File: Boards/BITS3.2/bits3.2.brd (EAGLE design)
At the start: 45 x 49.7 mm, 33 parts, among them U1 LMR16020, X1 53261-04, X2 53398-10

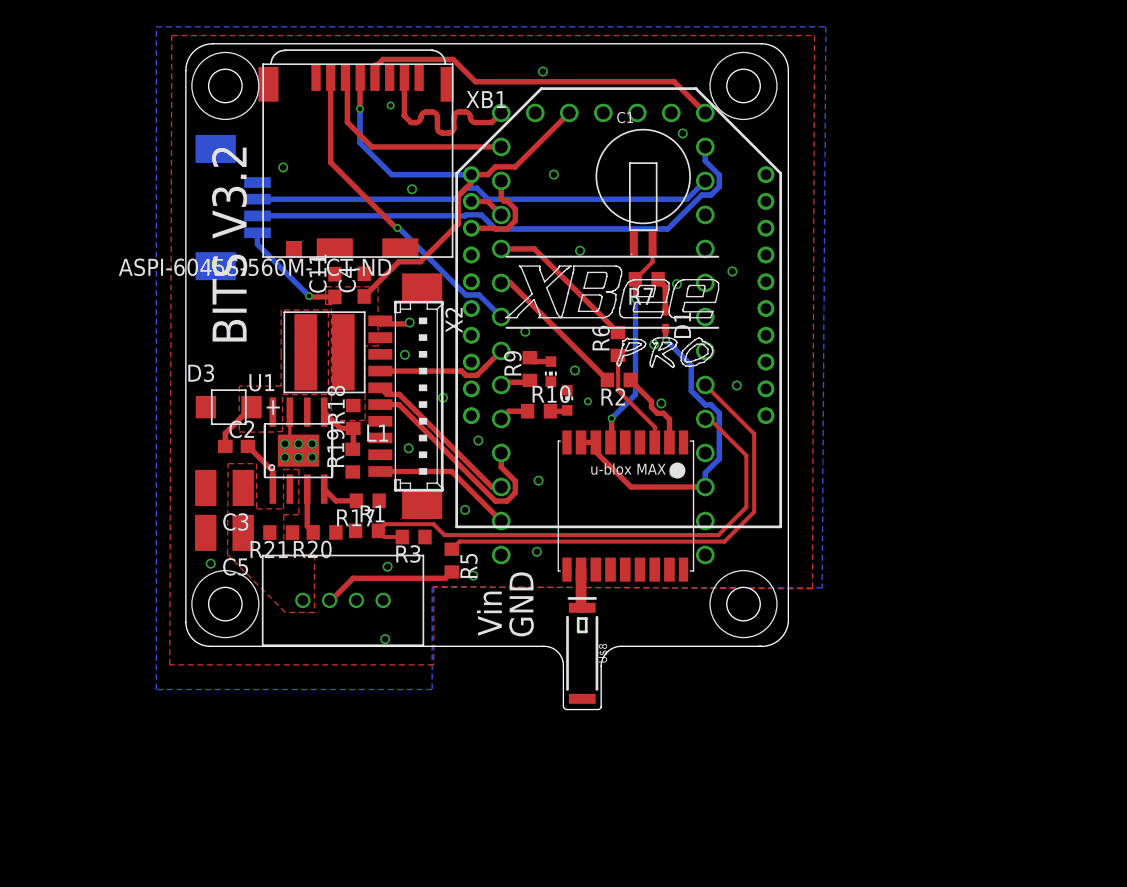
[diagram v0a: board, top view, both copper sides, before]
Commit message: Finalizing BITS v3.2
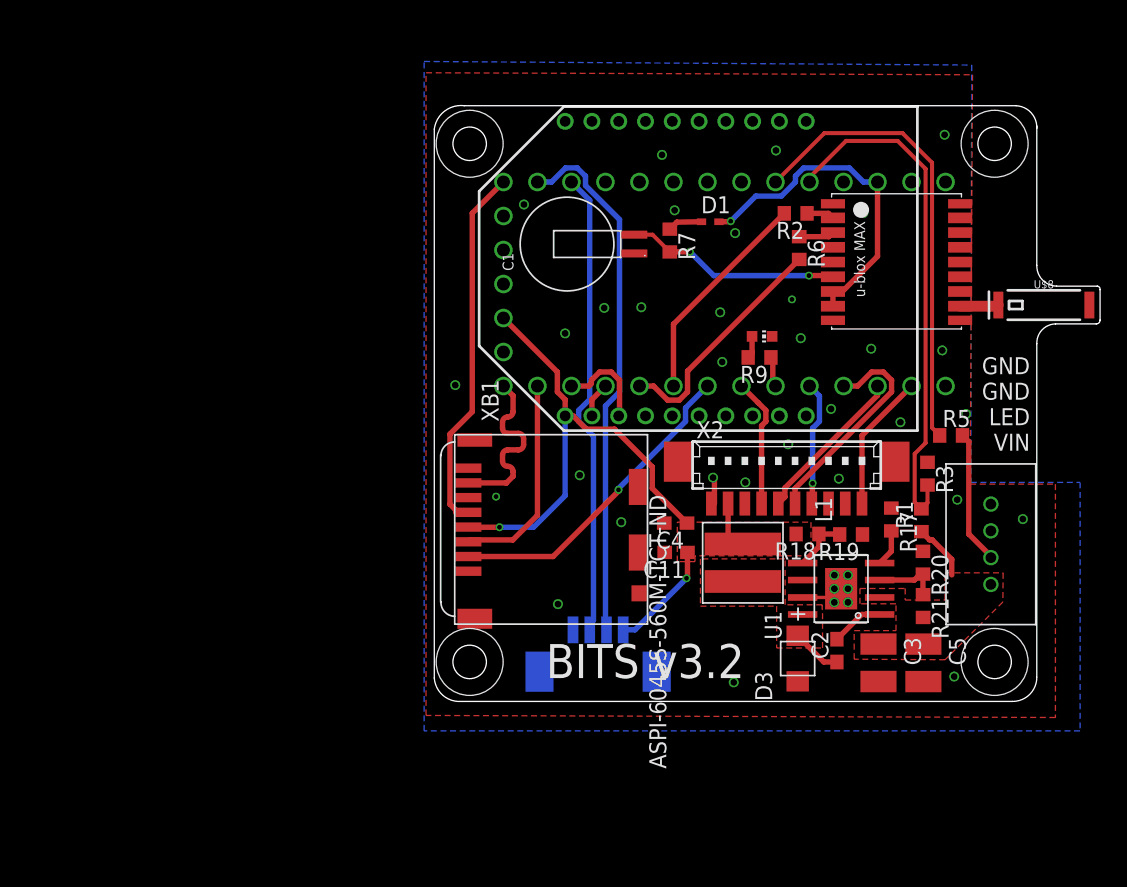
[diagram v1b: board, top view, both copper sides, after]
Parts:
- removed LED2: Green, led:CHIP-LED0603
- removed R10: 470, resistor:R0603
- moved C5 53.1 mm to (55.3, -1.24), turned to 270 degrees
- moved C3 50.6 mm to (51.9, -1.23), turned to 270 degrees
- moved U$1 48.6 mm to (60.3, 7.62), turned to 90 degrees
- moved R21 48.3 mm to (55.3, 3.01), turned to 270 degrees
- moved C2 47.4 mm to (48.8, -0.32), turned to 90 degrees
- moved D3 46.5 mm to (45.9, -0.92), turned to 90 degrees
- moved R20 44.7 mm to (55.3, 6.24), turned to 270 degrees
- moved X1 44.0 mm to (31.0, -1.27), turned to 180 degrees
- moved U$8 43.2 mm to (64.3, 25.5), turned to 0 degrees
- moved U1 41.8 mm to (49.1, 4.30), turned to 90 degrees
- moved R1 41.4 mm to (55.1, 9.41), turned to 90 degrees
- moved R17 39.1 mm to (52.9, 9.47), turned to 270 degrees
- moved R3 38.7 mm to (55.6, 12.9), turned to 270 degrees
- moved R5 38.4 mm to (57.4, 15.7), turned to 0 degrees
- moved R19 37.6 mm to (49.9, 8.35), turned to 180 degrees
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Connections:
- removed net LED2: R10.1, U$2.3
- removed net N$5: LED2.A, R10.2
- net GND: no longer LED2.C
- net NETAV: now also U$2.3
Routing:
- net NETAV: track 0.00 -> 9.32 mm, vias 0 -> 1
- net TX3: track 11.3 -> 17.6 mm
- net RX3: track 10.9 -> 16.3 mm
- net N$3: track 7.66 -> 2.65 mm
- net +3V3: track 70.3 -> 74.5 mm
- net N$4: track 6.15 -> 2.07 mm
- net IN1: track 0.28 -> 4.28 mm
- net LED2: track 2.21 -> 0.00 mm
- net N$7: track 2.79 -> 4.96 mm
- net N$5: track 1.28 -> 0.00 mm
- net GND: track 4.98 -> 4.73 mm, vias 34 -> 38
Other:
- board size 45 x 49.7 mm -> 49.7 x 44.5 mm
- board text added: "2S LiPo"
- board text added: "3V3>"
- board text added: "</CMD>"
- board text added: "BITS v3.2"
- board text added: "BPP"
- board text added: "GND GND LED VIN"
- board text added: "GND>"
- board text added: "Isolated Conn GND IN_B OUT_A 3V3"
- board text removed: "BITS V3.2"
- board text removed: "GND"
- board text removed: "Vin"
